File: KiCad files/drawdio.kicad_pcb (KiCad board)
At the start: 2 copper layers, 20 parts, among them J1 Jack, P1 CON1, P2 CON2, P3 PWR_SW, P4 SPK, P9 CONN_02X04, Q1 BC558, Q2 BC547, Q3 BC558, Q4 BC547, U1 NE555

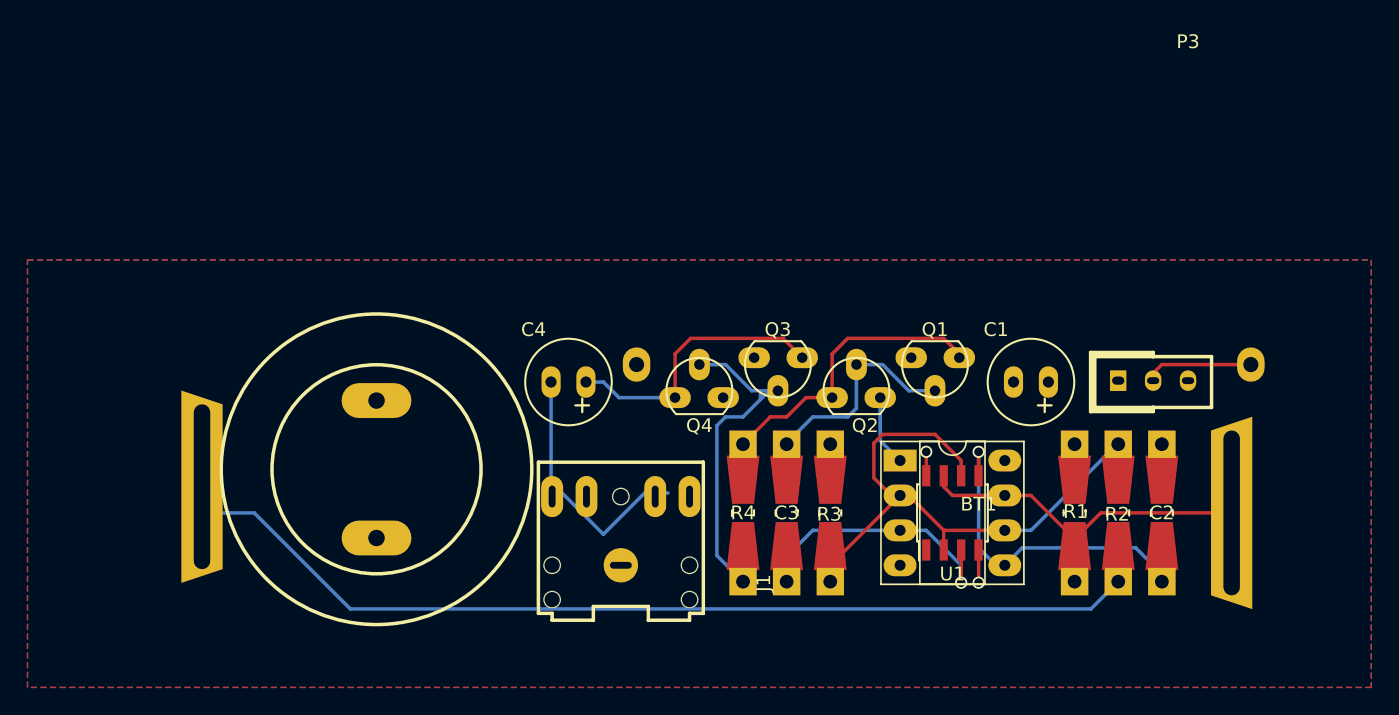
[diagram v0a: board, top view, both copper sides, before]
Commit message: Redimensionada
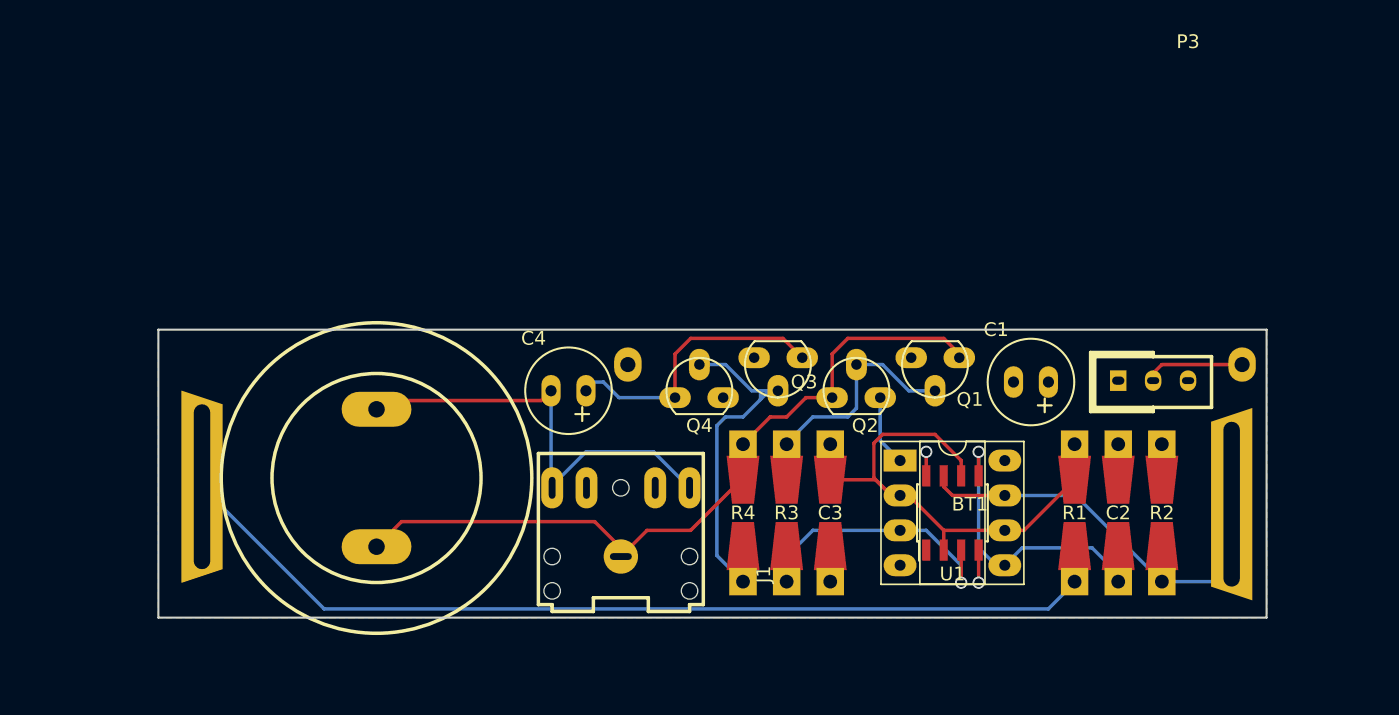
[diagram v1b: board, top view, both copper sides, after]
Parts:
- C2, C3, R1, R2, R3, R4: footprint Resistors_Universal:Resistor_SMD+THTuniversal_0805to1206_RM10_HandSoldering -> drawdio:Resistor_SMD+THTuniversal_0805to1206_RM10_HandSoldering
- moved R2 6.35 mm to (128.0, 90.2)
- moved C2 3.17 mm to (124.8, 90.2)
- moved R1 3.17 mm to (121.7, 90.2)
- moved BT1 0.64 mm to (111.5, 79.4)
- moved C4 0.64 mm to (86.1, 81.3)
- moved J1 0.64 mm to (88.6, 93.3)
- moved P2 0.64 mm to (133.1, 89.5)
- moved P4 0.63 mm to (70.9, 87.6)
- turned C3 to 270 degrees
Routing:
- net Net-(J1-Pad1): track 25.3 -> 57.4 mm
- net Net-(C4-Pad2): track 18.6 -> 35.2 mm
- net /pin2: track 48.0 -> 40.9 mm
- net /pin7: track 27.7 -> 34.2 mm
- net /pin5: track 27.8 -> 23.9 mm
- net Net-(P1-Pad1): track 74.2 -> 71.7 mm
- net GND: track 10.4 -> 11.6 mm
- net Net-(BT1-Pad1): track 7.91 -> 7.27 mm
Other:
- board outline added: 80.6 x 21 mm

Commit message: puede que funcione
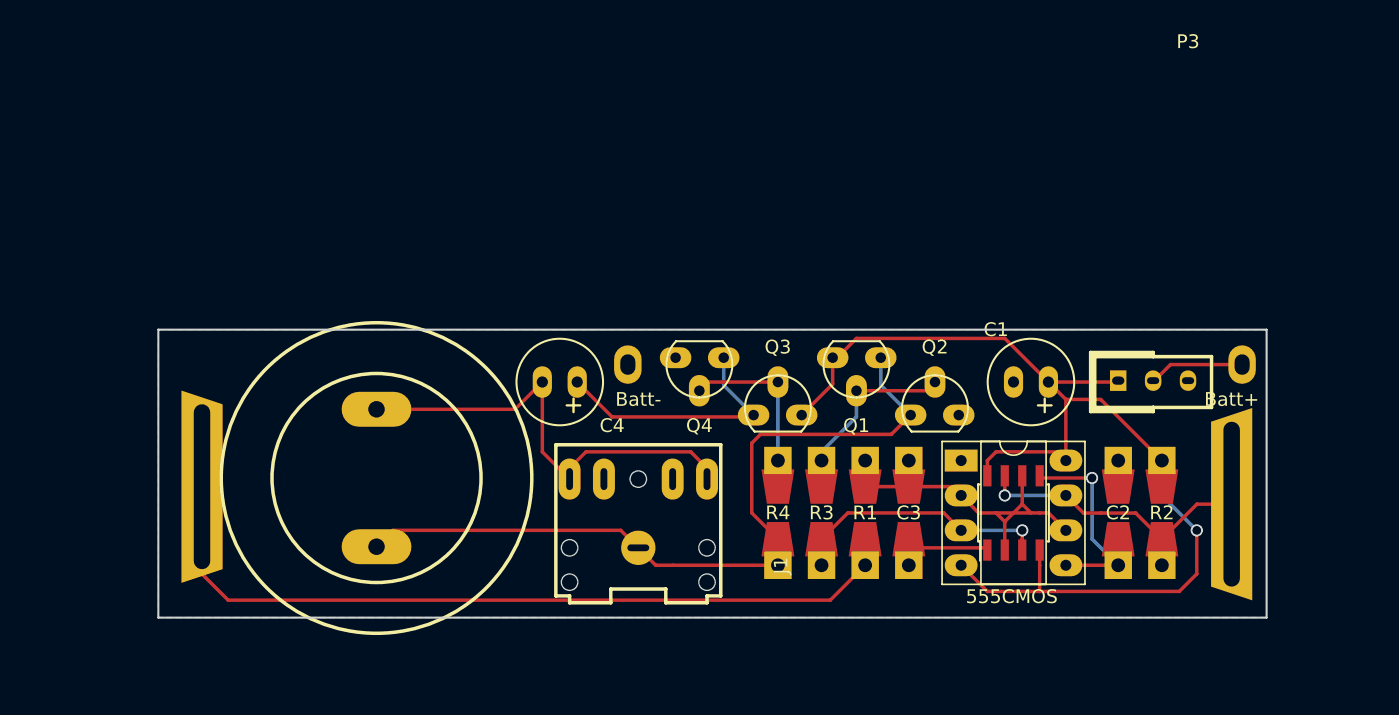
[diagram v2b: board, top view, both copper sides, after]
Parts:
- BT1: footprint drawdio:AAA_cell_holder -> AAA_cell_holder
- C2, C3, R1, R2, R3, R4: footprint drawdio:Resistor_SMD+THTuniversal_0805to1206_RM10_HandSoldering -> drawdio:Resistor_SMD+THT
- moved R1 15.2 mm to (106.4, 90.2)
- moved Q2 5.85 mm to (110.2, 82.5)
- moved C3 5.72 mm to (109.6, 90.2)
- moved Q1 5.71 mm to (107.1, 79.4)
- moved 555CMOS 4.45 mm to (113.4, 86.4)
- moved P9 4.45 mm to (117.2, 90.2)
- moved Q3 4.07 mm to (98.8, 82.5), turned to 0 degrees
- moved Q4 3.18 mm to (95.6, 79.4), turned to 180 degrees
- moved R3 2.54 mm to (103.3, 90.2)
- moved R4 2.54 mm to (100.1, 90.2), turned to 270 degrees
- moved J1 1.42 mm to (89.9, 92.7)
- moved C4 0.90 mm to (85.5, 80.6)
- renumbered U1 to 555CMOS
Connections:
- J1 pad 5: (no net) -> Net-(J1-Pad5)
- J1 pad 6: (no net) -> Net-(J1-Pad6)
- P3 pad 3: (no net) -> Net-(P3-Pad3)
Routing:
- net VCC: track 6.71 -> 80.8 mm, vias 2 -> 1
- net /pin2: track 40.9 -> 27.4 mm
- net Net-(P1-Pad1): track 71.7 -> 58.3 mm
- net Net-(Q3-Pad2): track 27.4 -> 14.5 mm
- net /pin7: track 34.2 -> 22.2 mm, vias 0 -> 1
- net /pin5: track 23.9 -> 16.7 mm
- net GND: track 11.6 -> 6.04 mm
- net Net-(Q1-Pad2): track 18.5 -> 13.1 mm
- net /pin3: track 22.6 -> 19.3 mm
- net Net-(J1-Pad1): track 57.4 -> 59.8 mm
- net Net-(C4-Pad1): track 21.0 -> 19.0 mm
- net Net-(C4-Pad2): track 35.2 -> 33.4 mm
- added copper zone on B.Cu, net GND
- removed copper zone on F.Cu, net GND
- removed copper zone on B.Cu, net VCC
